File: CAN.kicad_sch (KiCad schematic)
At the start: 7 parts, among them U6 TCAN334GD

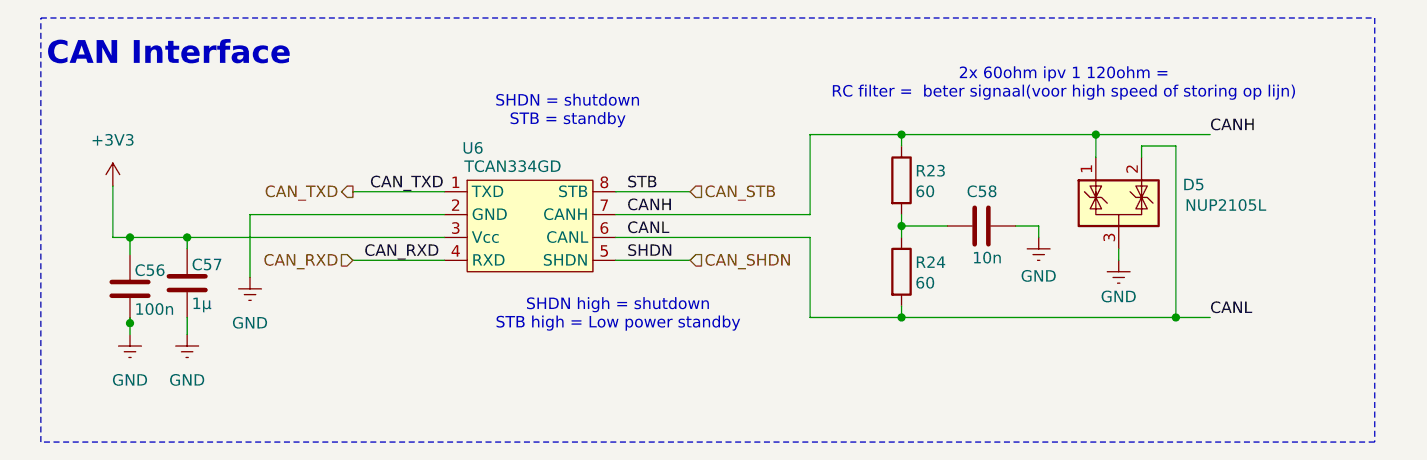
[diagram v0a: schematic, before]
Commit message: schema's finalized
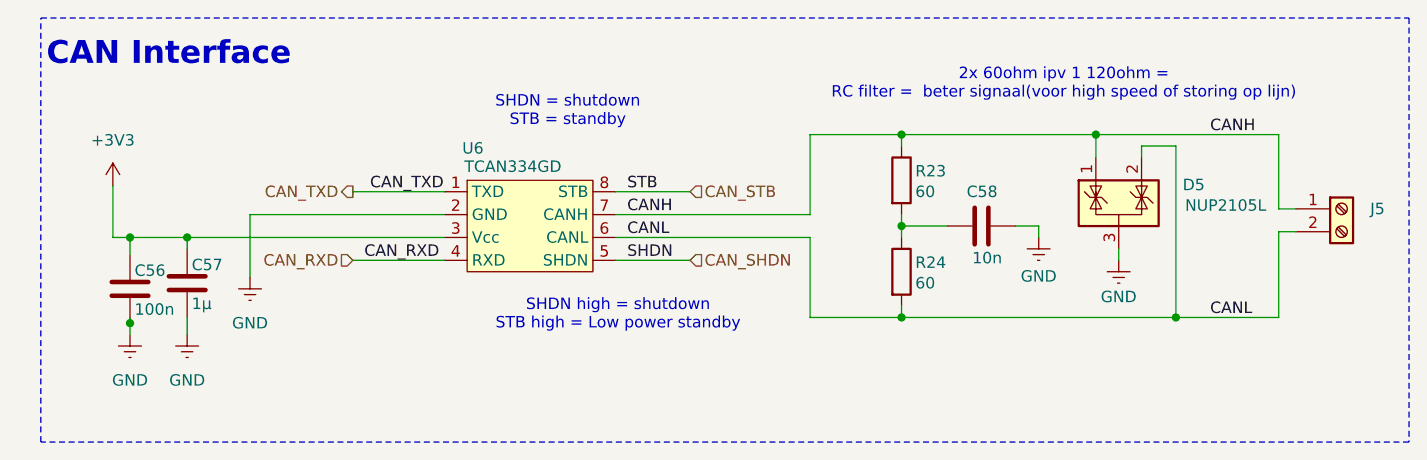
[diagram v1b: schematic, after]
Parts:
- added J5: Screw_Terminal_01x02, symbol Connector:Screw_Terminal_01x02
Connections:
- net CANH: now also J5.1 (Pin_1)
- net CANL: now also J5.2 (Pin_2)
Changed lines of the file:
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@@
 	(rectangle
 		(start 79.629 55.626)
-		(end 227.838 102.743)
+		(end 231.648 102.743)
 		(stroke
 			(width 0)
@@
 	(wire
 		(pts
+			(xy 217.17 79.375) (xy 217.17 88.9)
+		)
+		(stroke
+			(width 0)
+			(type default)
+		)
+	)
+	(wire
+		(pts
 			(xy 89.535 80.01) (xy 89.535 81.915)
 		)
@@
 	(wire
 		(pts
+			(xy 219.075 76.835) (xy 217.17 76.835)
+		)
+		(stroke
+			(width 0)
+			(type default)
+		)
+	)
+	(wire
+		(pts
 			(xy 114.3 82.55) (xy 124.46 82.55)
 		)
@@
 	(wire
 		(pts
+			(xy 217.17 76.835) (xy 217.17 68.58)
+		)
+		(stroke
+			(width 0)
+			(type default)
+		)
+	)
+	(wire
+		(pts
 			(xy 175.26 78.74) (xy 175.26 80.01)
 		)
@@
 	(wire
 		(pts
-			(xy 196.85 68.58) (xy 209.55 68.58)
+			(xy 196.85 68.58) (xy 217.17 68.58)
 		)
 		(stroke
@@
 	(wire
 		(pts
-			(xy 205.74 88.9) (xy 209.55 88.9)
+			(xy 205.74 88.9) (xy 217.17 88.9)
 		)
 		(stroke
@@
 		(pts
 			(xy 175.26 77.47) (xy 175.26 78.74)
+		)
+		(stroke
+			(width 0)
+			(type default)
+		)
+	)
+	(wire
+		(pts
+			(xy 219.075 79.375) (xy 217.17 79.375)
 		)
 		(stroke
@@
 					(unit 1)
 				)
+			)
+		)
+	)
+	(symbol
+		(lib_id "Connector:Screw_Terminal_01x02")
+		(at 224.155 76.835 0)
+		(unit 1)
+		(body_style 1)
+		(exclude_from_sim no)
+		(in_bom yes)
+		(on_board yes)
+		(in_pos_files yes)
+		(dnp no)
+		(fields_autoplaced yes)
+		(property "Reference" "J5"
+			(at 227.33 76.8349 0)
+			(show_name no)
+			(do_not_autoplace no)
+			(effects
+				(font
+					(size 1.27 1.27)
+				)
+				(justify left)
+			)
+		)
+		(property "Value" "Screw_Terminal_01x02"
+			(at 227.33 79.3749 0)
+			(hide yes)
+			(show_name no)
+			(do_not_autoplace no)
+			(effects
+				(font
+					(size 1.27 1.27)
+				)
+				(justify left)
+			)
+		)
+		(property "Footprint" ""
+			(at 224.155 76.835 0)
+			(hide yes)
+			(show_name no)
+			(do_not_autoplace no)
+			(effects
+				(font
+					(size 1.27 1.27)
+				)
+			)
+		)
+		(property "Datasheet" ""
+			(at 224.155 76.835 0)
+			(hide yes)
+			(show_name no)
+			(do_not_autoplace no)
+			(effects
+				(font
+					(size 1.27 1.27)
+				)
+			)
+		)
+		(property "Description" "Generic screw terminal, single row, 01x02, script generated (kicad-library-utils/schlib/autogen/connector/)"
+			(at 224.155 76.835 0)
+			(hide yes)
+			(show_name no)
+			(do_not_autoplace no)
+			(effects
+				(font
+					(size 1.27 1.27)
+				)
+			)
+		)
+		(pin "1"
+		)
+		(pin "2"
+		)
+		(instances
+			(project "ESC_PLC"
+				(path "/5bd3bb6f-fe53-443c-806c-077e2bbb5d14/fe40b710-6ad0-4f5f-80cc-5572b327525f"
+					(reference "J5")
+					(unit 1)
+				)
